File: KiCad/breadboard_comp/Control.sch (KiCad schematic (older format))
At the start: 89 parts, among them SW8 SW_Push, U2 74LS04, U28 74LS08, U38 74LS08, U57 74LS04, U66 74LS04, U85 74LS08, U86 74LS04, U88 74LS161, U89 74LS138, U90 28C256, U91 28C256, U92 74LS04, U93 28C256, U94 28C256, U95 74LS04, U96 74LS04

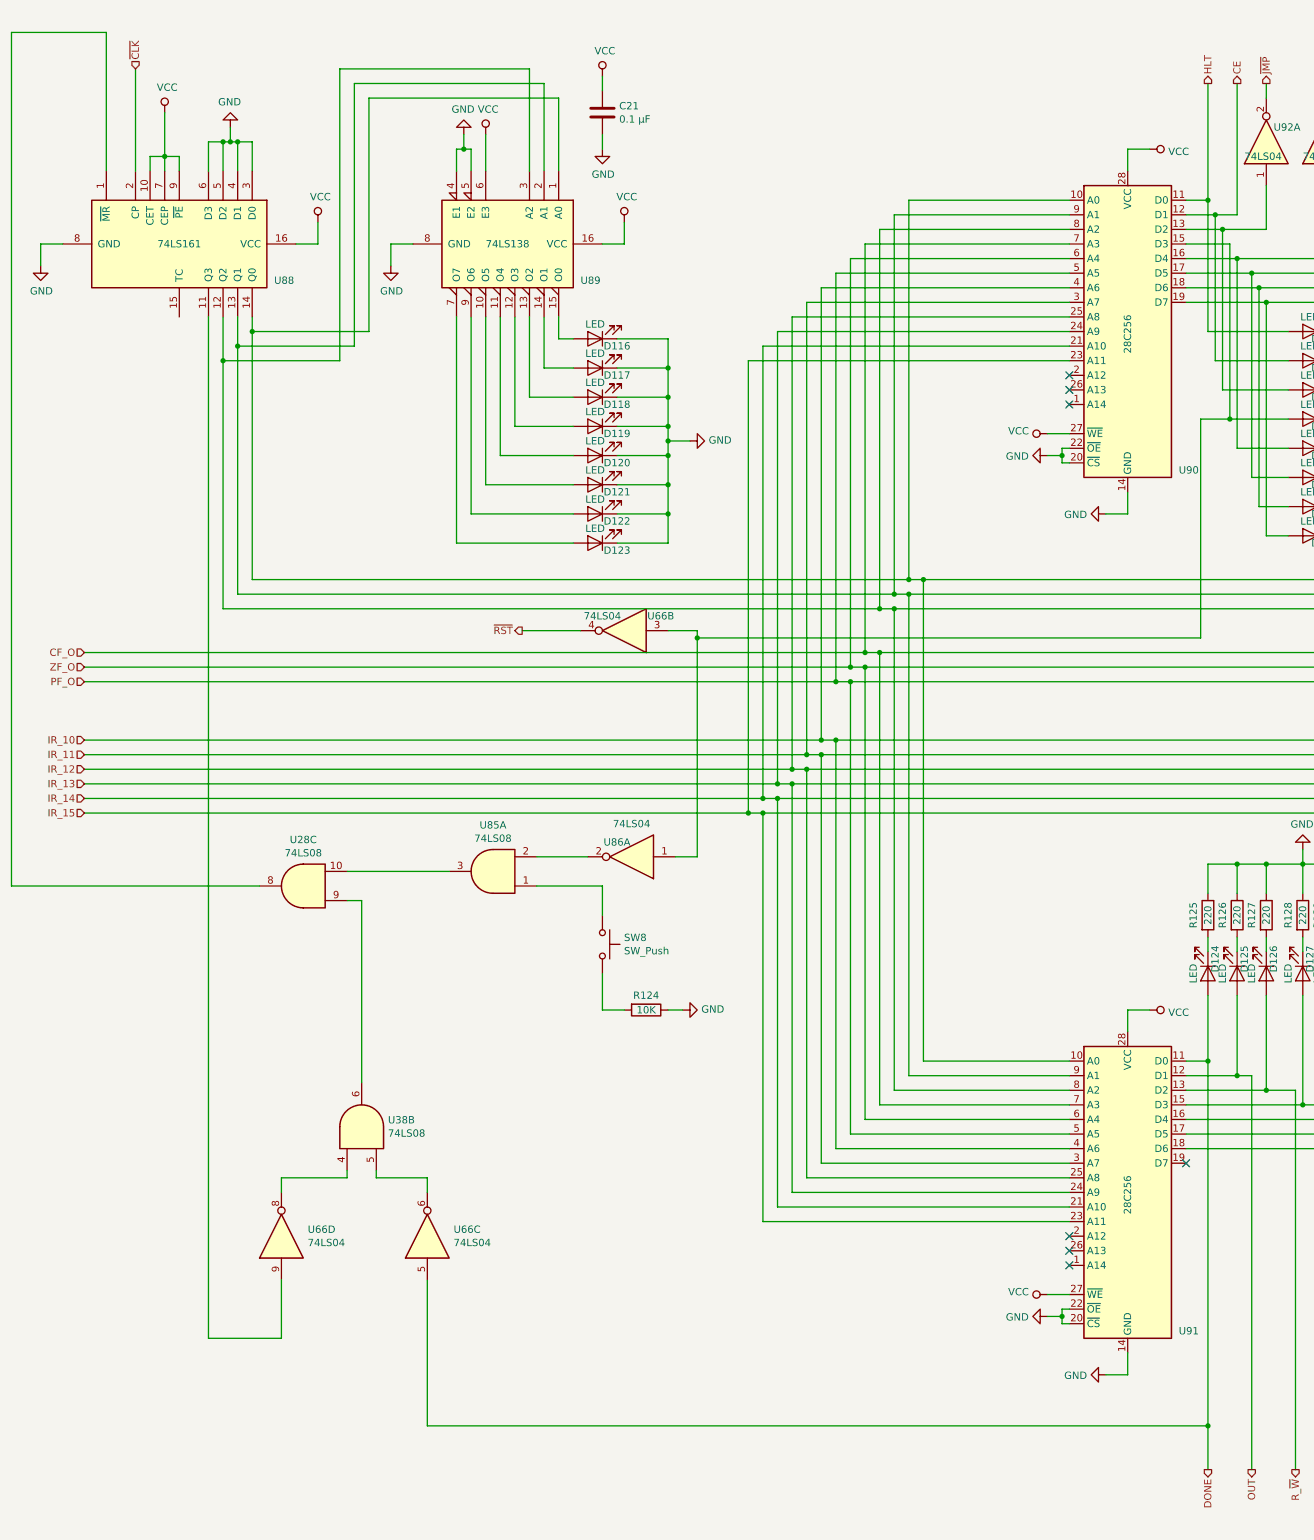
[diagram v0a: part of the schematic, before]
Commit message: Schematic + Report Progress
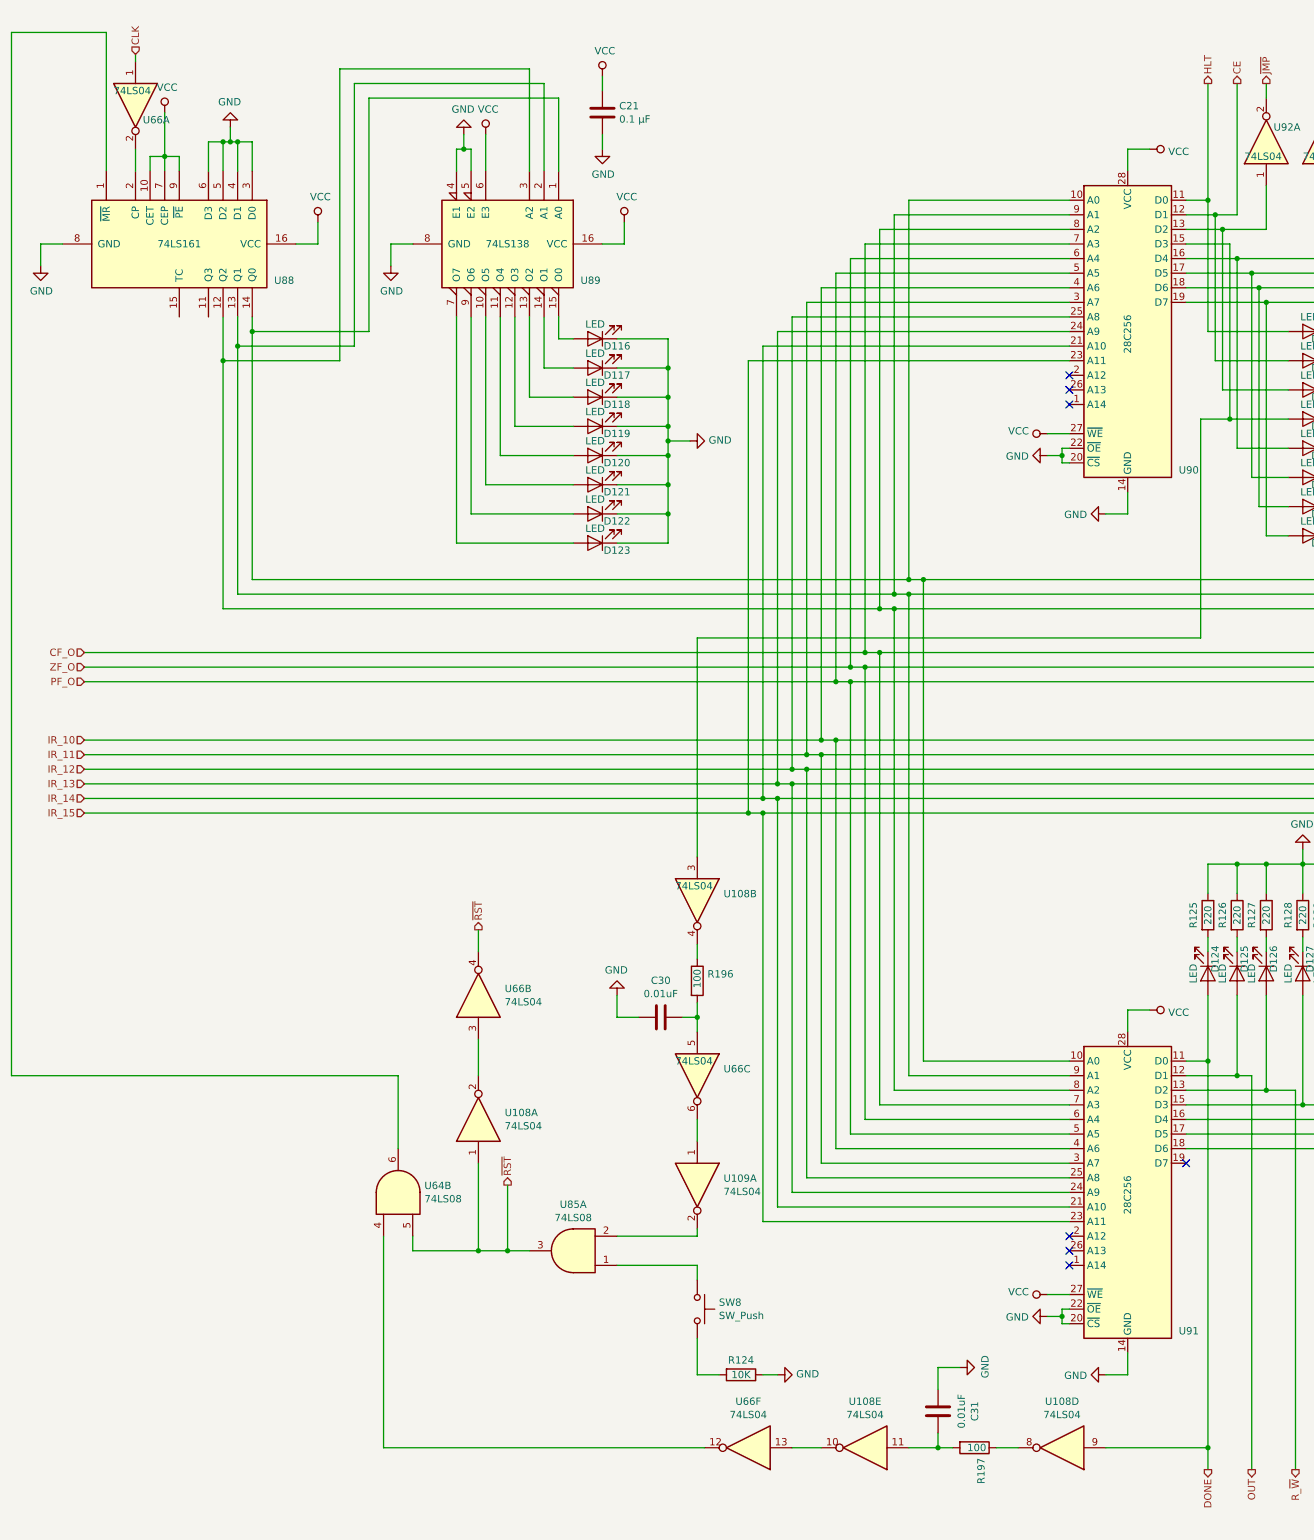
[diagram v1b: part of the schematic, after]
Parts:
- removed U28, U38: 74LS08, symbol 74xx:74LS08
- removed unit 4 of U66
- removed U86: 74LS04, symbol 74xx:74LS04
- added C30, C31: 0.01uF, symbol Device:C
- added R196, R197: 100, symbol Device:R
- added U108, U109: 74LS04, symbol 74xx:74LS04
- added U64: 74LS08, symbol 74xx:74LS08
- added unit 1 of U66
- added unit 6 of U66
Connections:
- net DONE: now also U108.9; no longer U66.5
- net GND: now also C30.2, C31.2
- net ~RST: now also U85.3, U108.1, U64.5
- net at U85.2: now also U109.2
- net at D131.2 (A), U90.15 (D3): now also U108.3; no longer U66.3
- net at U66.6: now also U109.1
- net at U88.1 (~MR): now also U64.6
- net ~CLK: no longer names the net of U88.2 (CP)
- net ~CLK: now also U66.2
- new net: R196.1, U108.4
- new net: C30.1, R196.2, U66.5
- new net: R197.1, U108.8
- new net: U108.10, U66.13
- new net: C31.1, R197.2, U108.11
- new net: U64.4, U66.12
- new net: U108.2, U66.3
- new net CLK: U66.1
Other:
- moved on the sheet: R124, SW8, U85A
